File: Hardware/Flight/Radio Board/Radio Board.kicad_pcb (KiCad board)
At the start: 2 copper layers, 80 x 80 mm, 11 parts, among them J1 Conn_01x20_Female, J2 Conn_Coaxial, J3 Conn_Coaxial, U1 RFM95W-915S2, U2 RFM95W-915S2

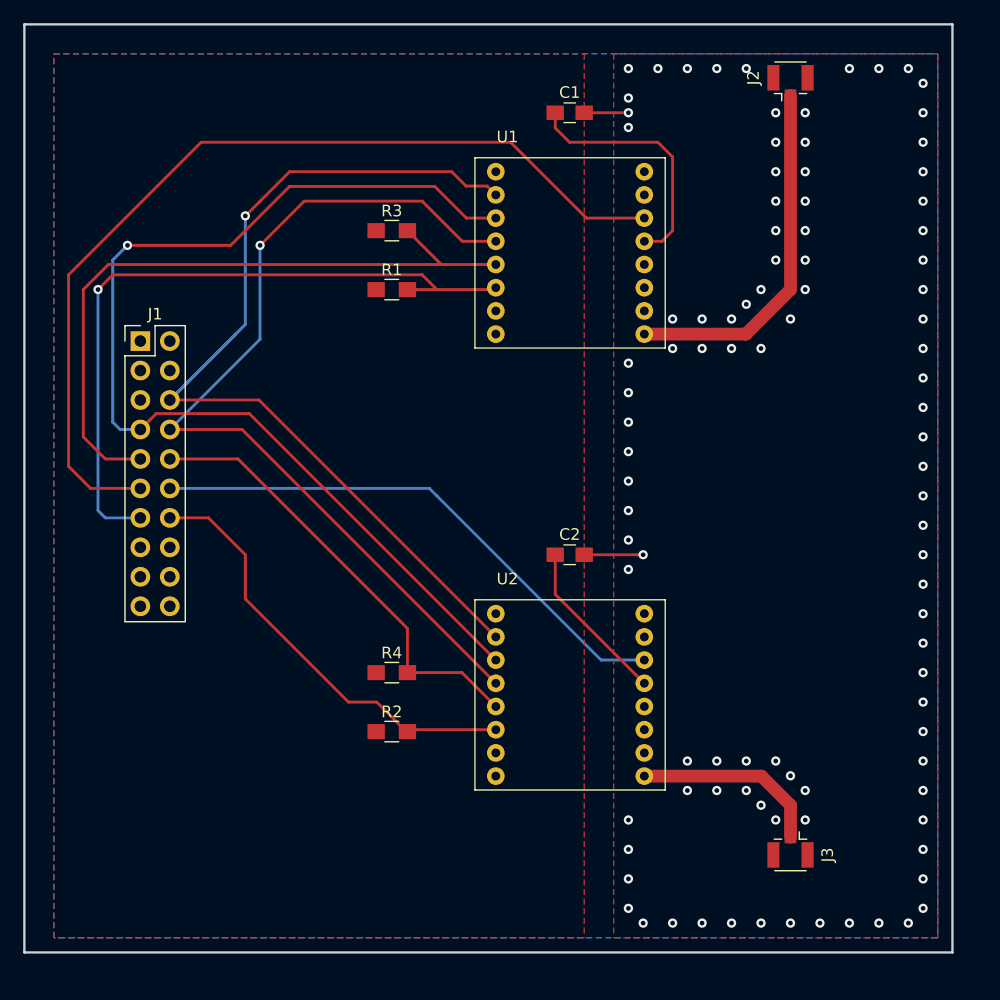
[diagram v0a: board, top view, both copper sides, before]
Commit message: radio board for review
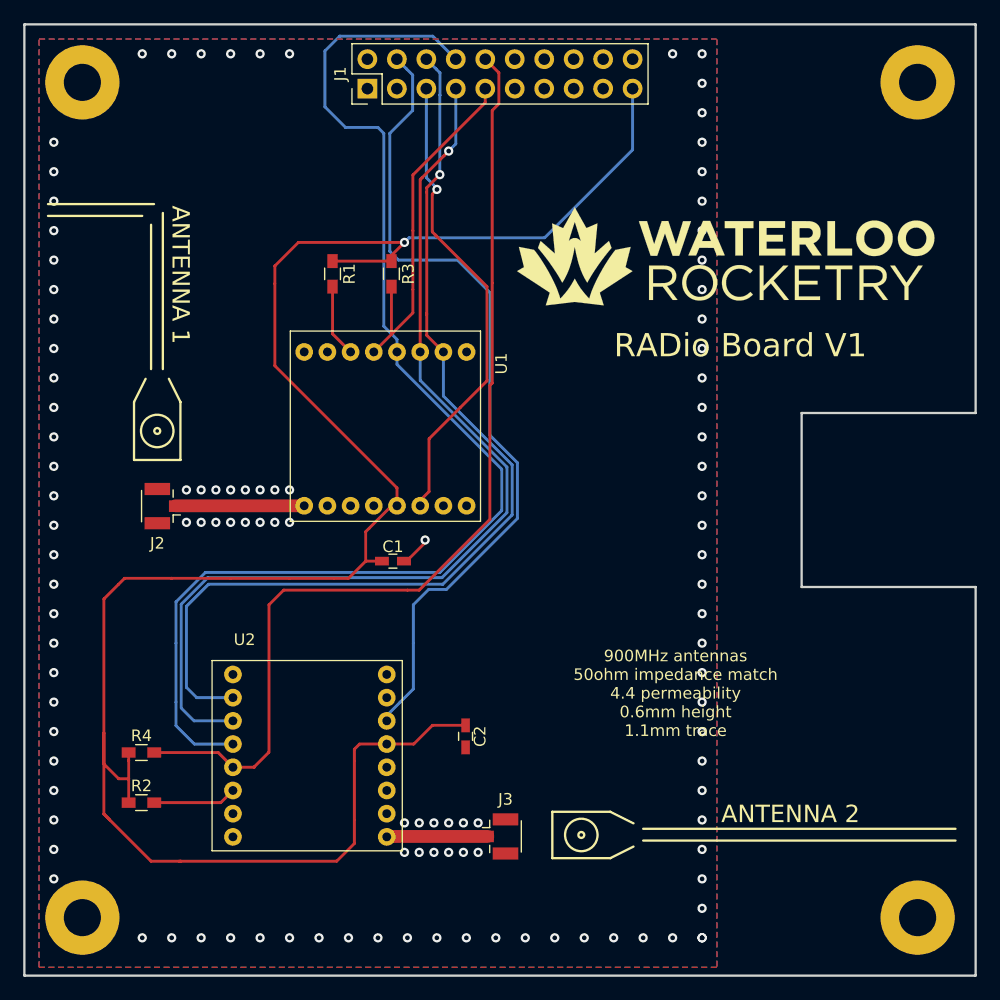
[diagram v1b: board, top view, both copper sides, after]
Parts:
- added G***: LOGO, Team_Logo:Logo_Horizontal_Silkscreen_10mm, F.Cu at (60.5, 20.0)
- added REF**: MountingHole_3.2mm_M3_Pad, Mounting_Holes:MountingHole_3.2mm_M3_Pad, F.Cu at (5.00, 77.0)
- added REF**: MountingHole_3.2mm_M3_Pad, Mounting_Holes:MountingHole_3.2mm_M3_Pad, F.Cu at (5.00, 5.00)
- added REF**: MountingHole_3.2mm_M3_Pad, Mounting_Holes:MountingHole_3.2mm_M3_Pad, F.Cu at (77.0, 77.0)
- added REF**: MountingHole_3.2mm_M3_Pad, Mounting_Holes:MountingHole_3.2mm_M3_Pad, F.Cu at (77.0, 5.00)
- C1, C2: footprint Capacitors_SMD:C_0805_HandSoldering -> Capacitors_SMD:C_0603_HandSoldering
- R1, R2, R3, R4: footprint Resistors_SMD:R_0805_HandSoldering -> Resistors_SMD:R_0603_HandSoldering
- U1, U2: footprint RF_Modules:Hopref_RFM9XW_THT -> Payload_Radios:Hopref_RFM9XW_THT
- moved J2 65.2 mm to (11.9, 41.5), turned to 180 degrees
- moved C1 41.5 mm to (31.8, 46.3)
- moved J1 29.3 mm to (29.6, 5.54), turned to 90 degrees
- moved J3 25.1 mm to (41.0, 70.0), turned to 0 degrees
- moved U2 23.3 mm to (18.0, 56.0)
- moved R4 22.7 mm to (10.1, 62.8)
- moved R2 22.4 mm to (10.1, 67.1)
- moved C2 18.0 mm to (38.0, 61.4), turned to 270 degrees
- moved U1 15.7 mm to (38.1, 28.2), turned to 270 degrees
- moved R1 5.28 mm to (26.6, 21.5), turned to 270 degrees
- moved R3 3.73 mm to (31.6, 21.5), turned to 270 degrees
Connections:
- J1 pad 11: INT1 -> Net-(J1-Pad11)
- J1 pad 12: INT2 -> Net-(J1-Pad12)
- J1 pad 13: RST1 -> Net-(J1-Pad13)
- J1 pad 14: RST2 -> Net-(J1-Pad14)
- J1 pad 4: Net-(J1-Pad4) -> INT2
- J1 pad 5: Net-(J1-Pad5) -> INT1
- R1 pad 2: RST1 -> Net-(R1-Pad2)
- R2 pad 2: RST2 -> Net-(R2-Pad2)
- U1 pad 6: RST1 -> Net-(R1-Pad2)
- U2 pad 6: RST2 -> Net-(R2-Pad2)
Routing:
- net +3V3: track 35.9 -> 174.7 mm, vias 0 -> 1
- net RST1: track 60.9 -> 0.00 mm, vias 1 -> 0
- net CS2: track 39.2 -> 86.3 mm
- net INT1: track 80.6 -> 40.6 mm, vias 0 -> 1
- net RST2: track 38.0 -> 0.00 mm
- net CS1: track 59.0 -> 30.8 mm
- net SCK: track 79.6 -> 107.8 mm, vias 1 -> 0
- net INT2: track 47.0 -> 71.7 mm
- net Net-(J2-Pad1): track 30.9 -> 11.2 mm
- net Net-(J3-Pad1): track 16.4 -> 8.78 mm
- net Net-(R2-Pad2): track 0.00 -> 7.22 mm
- net MOSI: track 93.4 -> 86.2 mm
- net Net-(R1-Pad2): track 0.00 -> 6.28 mm
- net GND: track 8.89 -> 2.71 mm, vias 98 -> 113
- net MISO: track 87.2 -> 86.1 mm
- removed copper zone on F.Cu, net +3V3
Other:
- board size 80 x 80 mm -> 82 x 82 mm
- board text added: "900MHz antennas 50ohm impedance match 4.4 permeability 0.6mm height 1.1mm trace"
- board text added: "ANTENNA 1"
- board text added: "ANTENNA 2"
- board text added: "RADio Board V1"
